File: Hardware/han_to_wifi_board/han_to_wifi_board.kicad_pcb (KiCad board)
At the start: 2 copper layers, 34.1 x 47.8 mm, 35 parts, among them IC1 MIC2779L-2YM5_TR, IC3 MAX17644AATE+, J1 RJLSE4118101, J3 Conn_01x05_Male, SW1 RESET, U1 ESP-12F, U3 NCN5150

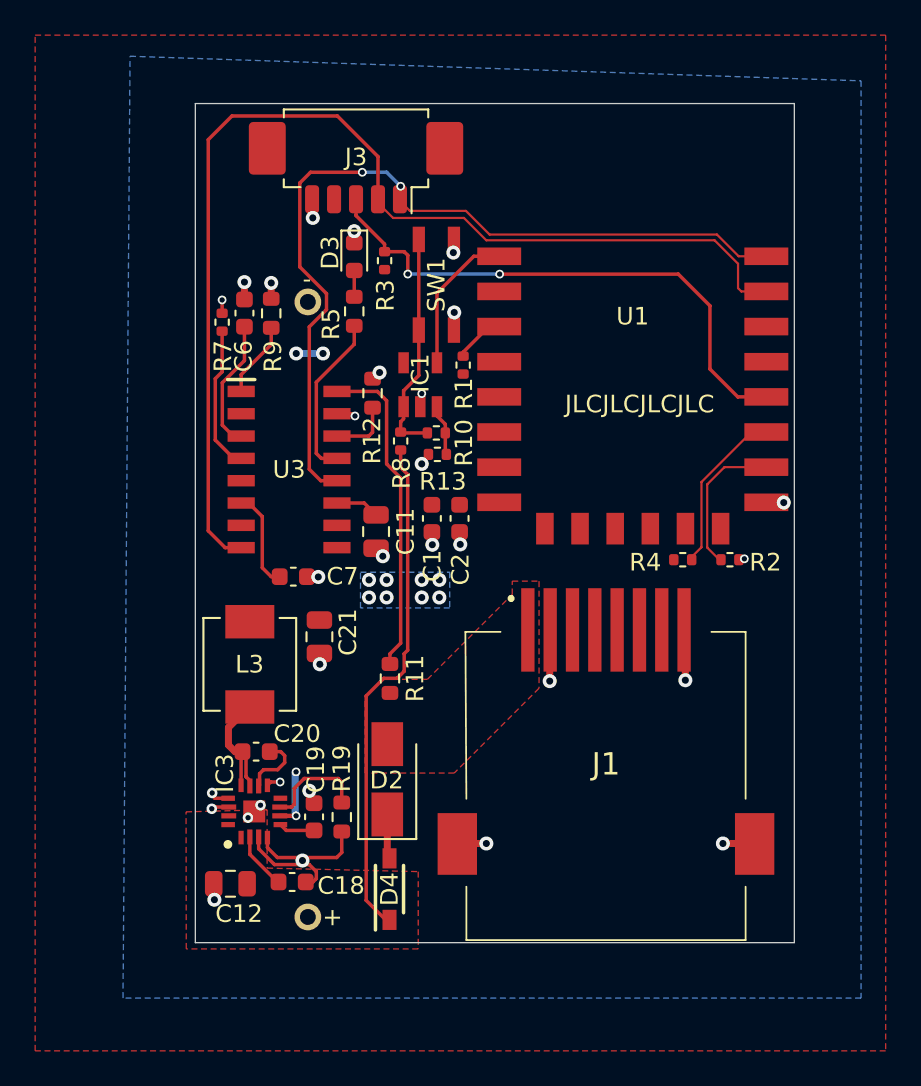
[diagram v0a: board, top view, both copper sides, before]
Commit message: September hw changes
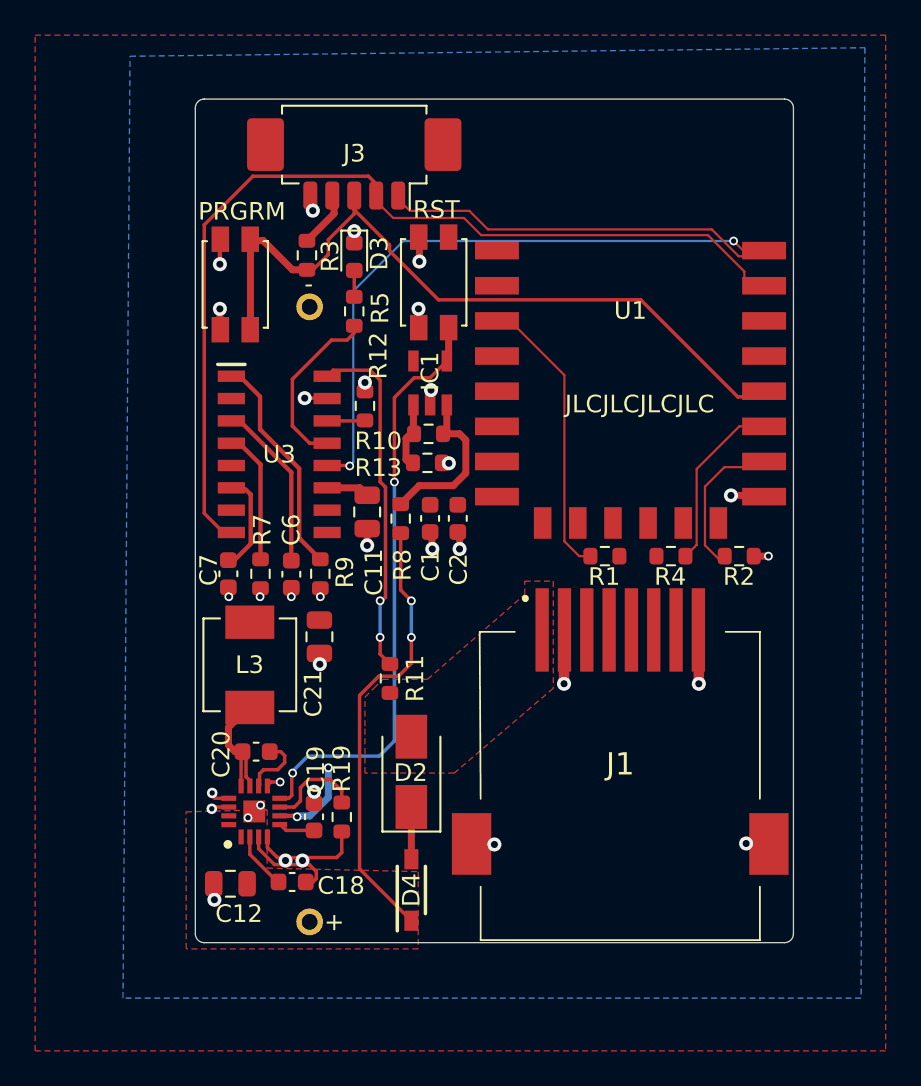
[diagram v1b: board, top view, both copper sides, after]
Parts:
- removed SW1: RESET, Button_Switch_SMD:SW_SPST_EVQP2
- added PRGRM: PRGRM, Button_Switch_SMD:SW_SPST_EVQP2, F.Cu at (117.6, 35.2)
- added RST: RESET, Button_Switch_SMD:SW_SPST_EVQP2, F.Cu at (128.9, 35.1)
- R1, R10, R13, R2, R3, R4, R7, R8: footprint Resistor_SMD:R_0402_1005Metric -> Resistor_SMD:R_0603_1608Metric
- moved C6 15.1 mm to (120.8, 51.7), turned to -90 degrees
- moved R9 15.1 mm to (122.4, 51.7), turned to -90 degrees
- moved R7 14.5 mm to (119.0, 51.7), turned to -90 degrees
- moved R1 13.5 mm to (138.6, 50.6), turned to 0 degrees
- moved R3 4.43 mm to (121.7, 33.5), turned to -90 degrees
- moved R8 4.42 mm to (127.0, 48.5), turned to 90 degrees
- moved C7 3.70 mm to (117.2, 51.7), turned to 90 degrees
- moved D2 1.44 mm to (127.6, 62.9)
- moved D4 1.25 mm to (127.6, 69.6)
- moved C11 1.23 mm to (125.1, 48.1)
- moved U3 1.03 mm to (120.1, 44.9)
- moved R12 0.84 mm to (125.0, 42.1)
- moved J1 0.81 mm to (139.5, 62.5)
- moved R13 0.74 mm to (128.5, 45.3)
- moved R4 0.70 mm to (142.4, 50.6)
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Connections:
- IC3 pad 8: unconnected-(IC3-Pad8) -> /~{RST}
- R13 pad 1: GND -> Net-(IC1-Pad1)
- R13 pad 2: Net-(IC1-Pad3) -> GND
- R8 pad 1: Net-(IC1-Pad1) -> /24V
- R8 pad 2: /24V -> Net-(IC1-Pad3)
- U1 pad 1: /~{RST} -> unconnected-(U1-Pad1)
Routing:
- net /~{RST}: track 8.37 -> 33.8 mm, vias 0 -> 2
- net Net-(R1-Pad1): track 2.88 -> 16.4 mm
- net /GPIO0: track 31.5 -> 42.6 mm, vias 2 -> 0
- net /ESP_Tx: track 47.7 -> 58.4 mm
- net /ESP_Rx: track 63.3 -> 53.2 mm
- net Net-(IC1-Pad1): track 12.9 -> 3.91 mm
- net Net-(R9-Pad1): track 4.33 -> 12.8 mm
- net GND: track 27.5 -> 34.7 mm, vias 30 -> 33
- net Net-(IC1-Pad3): track 2.93 -> 9.50 mm
- net /24V: track 29.0 -> 25.4 mm, vias 0 -> 2
- net +3V3: track 5.00 -> 8.05 mm, vias 12 -> 2
- net Net-(C6-Pad1): track 7.45 -> 9.64 mm
- net Net-(R11-Pad1): track 18.6 -> 20.0 mm, vias 0 -> 2
- net Net-(R12-Pad1): track 3.51 -> 2.16 mm
- net Net-(C7-Pad2): track 5.63 -> 4.89 mm
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- removed copper zone on B.Cu, net +3V3
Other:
- board size 34.1 x 47.8 mm -> 34 x 48 mm
- board text added: "AMS-utleser Nicholas Braaten September 2022"
- board text removed: "HAN-modul Nicholas Braaten Mai 2022"
